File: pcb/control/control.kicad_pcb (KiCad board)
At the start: 2 copper layers, 100 x 80 mm, 30 parts, among them J1 Barrel_Jack_MountingPin, J2 Screw_Terminal_01x02, SW1 OS102011MS2QN1, SW2 OS102011MS2QN1, U1 PicoW, U2 SN65HVD230DR, U3 FDN340P, U4 DMG2305UX-7

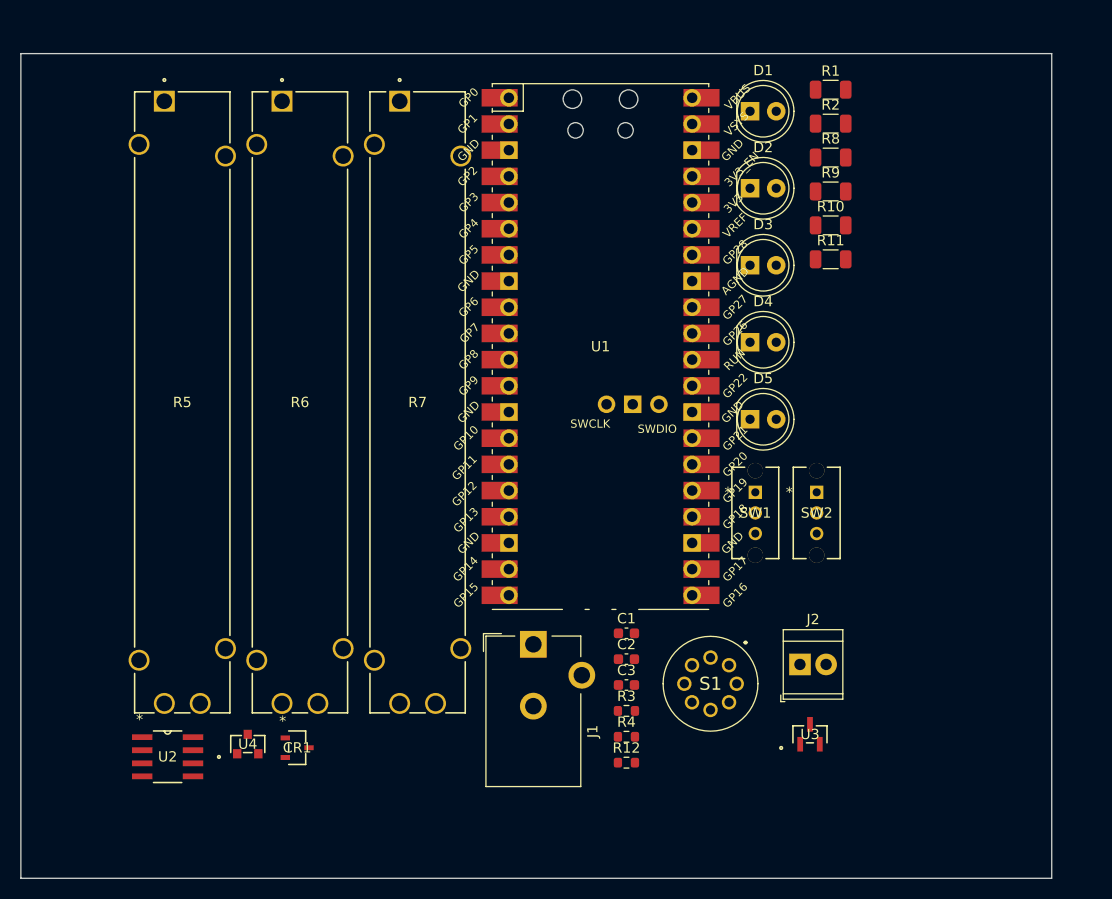
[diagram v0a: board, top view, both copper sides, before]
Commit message: Control PCB done
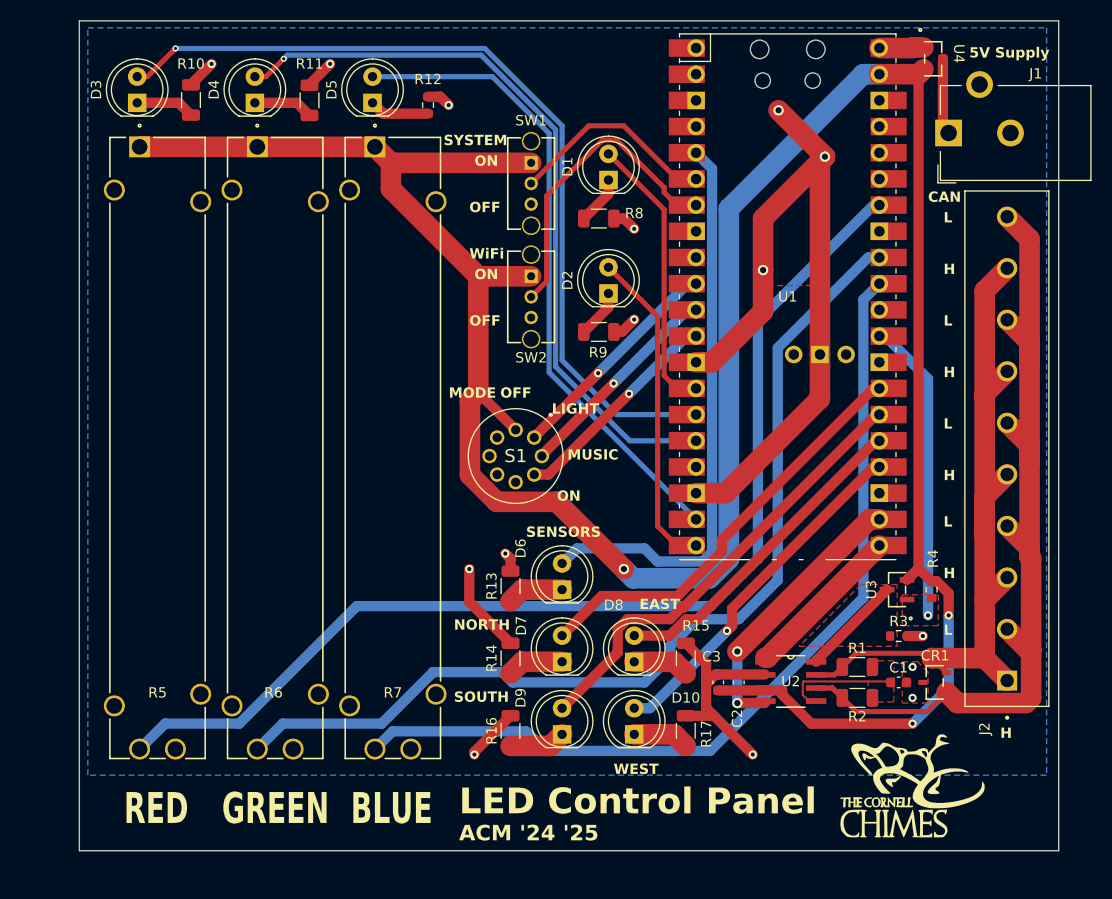
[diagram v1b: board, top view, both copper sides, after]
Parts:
- added D10: LED, LED_THT:LED_D5.0mm, F.Cu at (159.5, 126.0)
- added D6: LED, LED_THT:LED_D5.0mm, F.Cu at (152.5, 112.0)
- added D7: LED, LED_THT:LED_D5.0mm, F.Cu at (152.5, 119.0)
- added D8: LED, LED_THT:LED_D5.0mm, F.Cu at (159.5, 119.0)
- added D9: LED, LED_THT:LED_D5.0mm, F.Cu at (152.5, 126.0)
- added G***: LOGO, LOGO, F.Cu at (186.5, 131.0)
- added R13: 60Ω, Resistor_SMD:R_1206_3216Metric, F.Cu at (147.5, 111.7)
- added R14: 60Ω, Resistor_SMD:R_1206_3216Metric, F.Cu at (147.5, 118.7)
- added R15: 60Ω, Resistor_SMD:R_1206_3216Metric, F.Cu at (164.5, 118.7)
- added R16: 60Ω, Resistor_SMD:R_1206_3216Metric, F.Cu at (147.5, 125.7)
- added R17: 60Ω, Resistor_SMD:R_1206_3216Metric, F.Cu at (164.5, 125.7)
- J2: value Screw_Terminal_01x02 -> 1729092; footprint TerminalBlock_TE-Connectivity:TerminalBlock_TE_282834-2_1x02_P2.54mm_Horizontal -> 1729092:PHOENIX_1729092
- moved U4 94.0 mm to (188.5, 60.5), turned to -90 degrees
- moved R12 66.6 mm to (139.5, 65.0), turned to 90 degrees
- moved J1 63.9 mm to (190.0, 67.7), turned to 90 degrees
- moved R10 63.2 mm to (116.5, 64.5), turned to 90 degrees
- moved CR1 62.2 mm to (188.6, 121.0), turned to 180 degrees
- moved D3 61.5 mm to (111.3, 64.8), turned to 90 degrees
- moved U2 60.9 mm to (174.7, 120.9)
- moved R1 56.1 mm to (181.1, 119.5)
- moved R2 55.8 mm to (181.1, 122.5), turned to 180 degrees
- moved D4 53.4 mm to (122.7, 64.8), turned to 90 degrees
- moved R11 52.9 mm to (128.0, 64.5), turned to 90 degrees
- moved D5 47.8 mm to (134.1, 64.8), turned to 90 degrees
- moved SW1 38.7 mm to (149.5, 70.6)
- moved SW2 34.7 mm to (149.5, 81.6)
- moved R4 32.9 mm to (188.4, 112.0), turned to -90 degrees
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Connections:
- CR1 pad 1: /CANH -> /CANL
- CR1 pad 2: /CANL -> /CANH
- U1 pad 24: unconnected-(U1-GPIO18-Pad24)_1 -> /WFACE
- U1 pad 25: unconnected-(U1-GPIO19-Pad25) -> /EFACE
- U1 pad 26: unconnected-(U1-GPIO20-Pad26) -> /SFACE
- U1 pad 27: unconnected-(U1-GPIO21-Pad27)_1 -> /NFACE
- U1 pad 31: /POT_R -> /POT_B
- U1 pad 34: /POT_B -> /POT_R
- U1 pad 5: unconnected-(U1-GPIO3-Pad5)_1 -> /SENSORS
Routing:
- net VSYS: track 0.00 -> 259.8 mm, vias 0 -> 3
- net GND: track 0.00 -> 125.0 mm, vias 0 -> 15
- net /POT_R: track 0.00 -> 107.1 mm
- net /POT_G: track 0.00 -> 94.7 mm
- net /CANL: track 0.00 -> 88.3 mm
- net /POT_B: track 0.00 -> 86.1 mm
- net /LED_R: track 0.00 -> 83.4 mm, vias 0 -> 1
- net /CANH: track 0.00 -> 80.3 mm
- net /LED_G: track 0.00 -> 72.6 mm, vias 0 -> 1
- net /LED_B: track 0.00 -> 62.8 mm
- net /SENSORS: track 0.00 -> 55.4 mm
- net /SFACE: track 0.00 -> 43.9 mm
- net /NFACE: track 0.00 -> 41.4 mm
- net /WFACE: track 0.00 -> 34.5 mm, vias 0 -> 1
- net /EFACE: track 0.00 -> 31.6 mm
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- added copper zone on F.Cu, net /CAN_ENL
- added copper zone on F.Cu, net /CAN_RS
- added copper zone on F.Cu, net /CAN_VREF
- added copper zone on B.Cu, net GND
- added copper zone on F.Cu, net GND
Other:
- board size 100 x 80 mm -> 95 x 80.5 mm
- board text added: "5V Supply"
- board text added: "ACM '24 '25"
- board text added: "BLUE"
- board text added: "CAN"
- board text added: "EAST"
- board text added: "GREEN"
- board text added: "H"
- board text added: "L"
- board text added: "LED Control Panel"
- board text added: "LIGHT"
- board text added: "MODE"
- board text added: "MUSIC"
- board text added: "NORTH"
- board text added: "OFF"
- board text added: "ON"
- board text added: "RED"
- board text added: "SENSORS"
- board text added: "SOUTH"
- board text added: "SYSTEM"
- board text added: "WEST"
- board text added: "WiFi"
